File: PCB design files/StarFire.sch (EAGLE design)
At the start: 29 parts, among them U2 ATTINY85-20SU

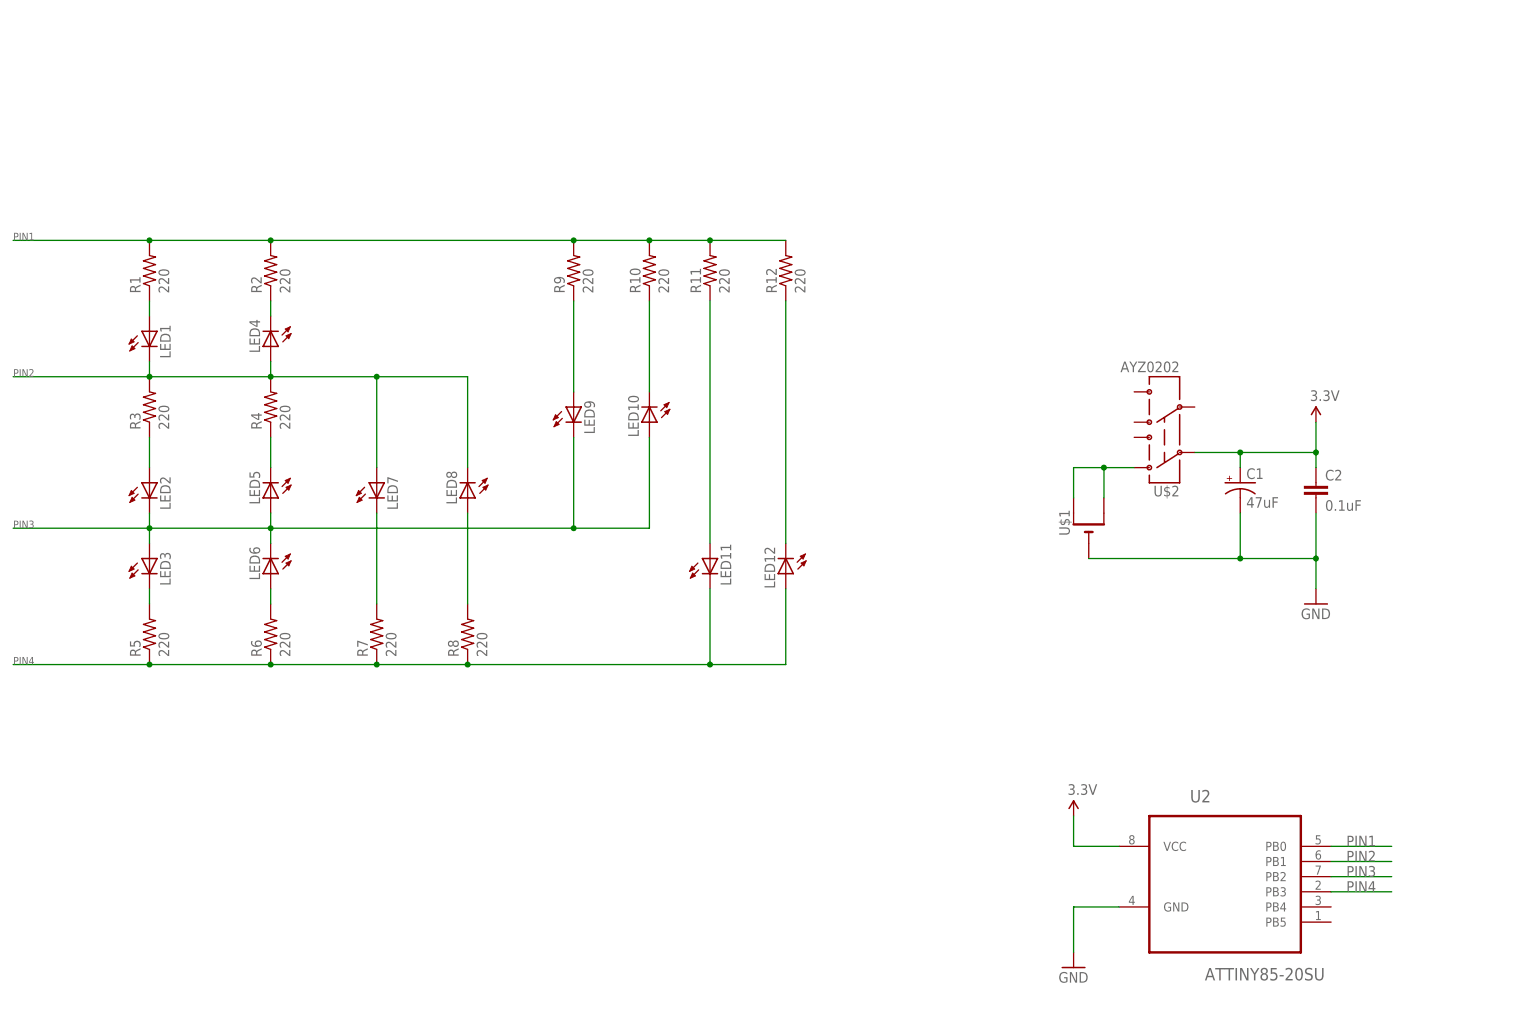
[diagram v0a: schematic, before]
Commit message: cleanup and sort
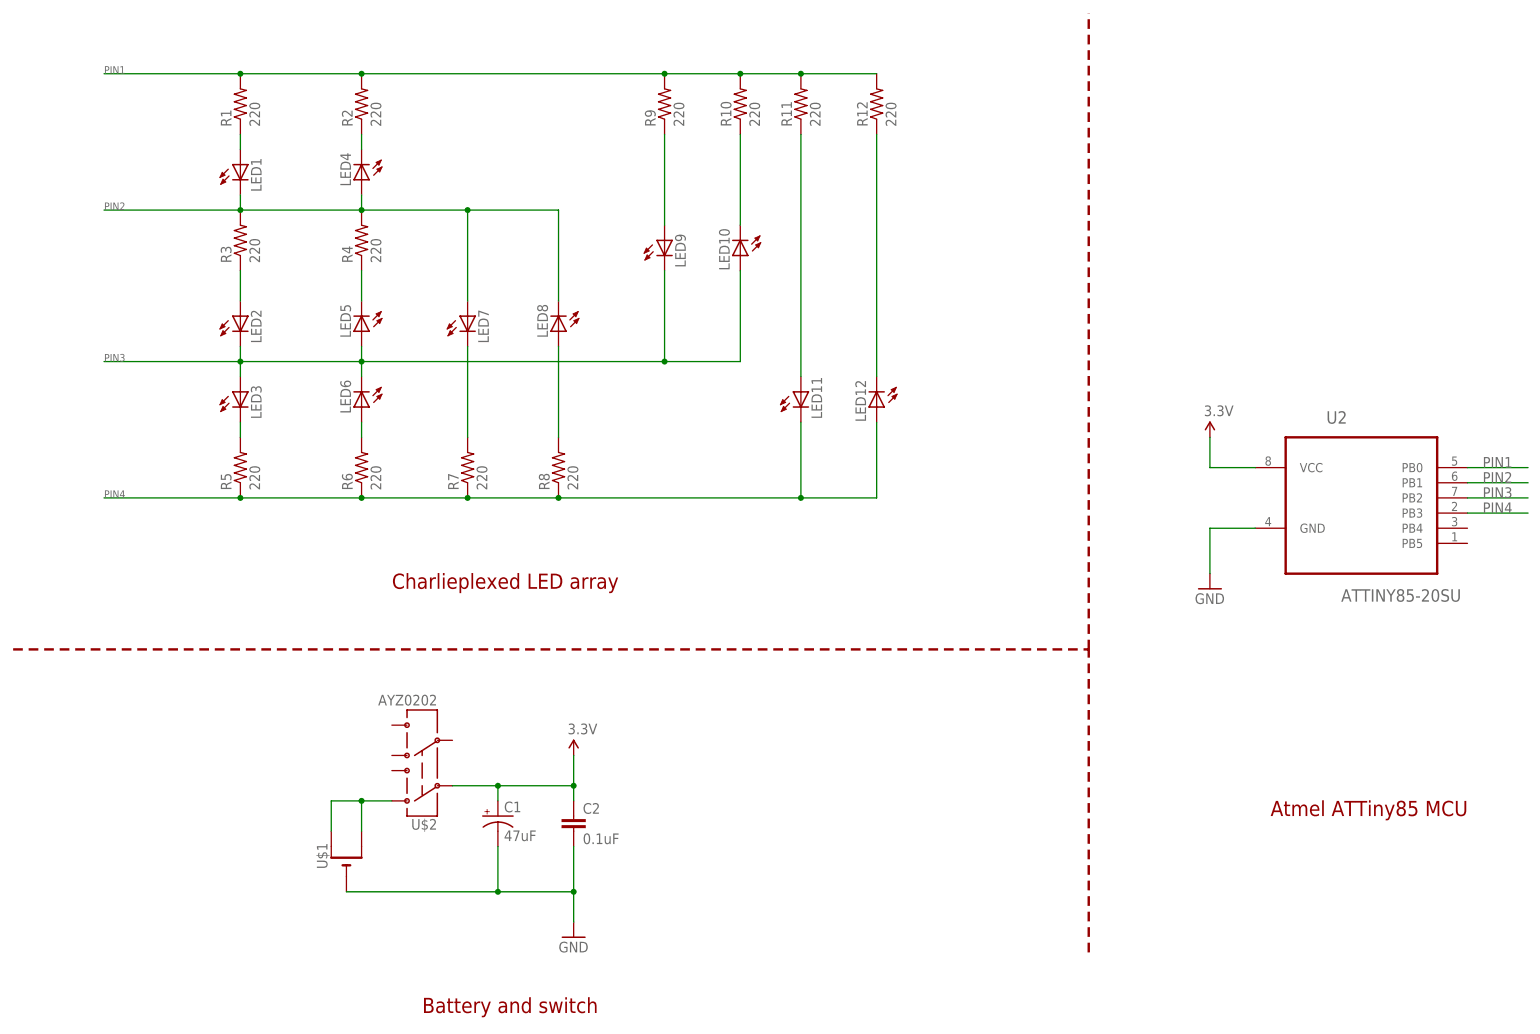
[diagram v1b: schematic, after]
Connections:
- net N$13: now also U$1.+1
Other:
- note added: "Atmel ATTiny85 MCU"
- note added: "Battery and switch"
- note added: "Charlieplexed LED array"
- moved on the sheet: C1, C2, LED1, LED10, LED11, LED12, LED2, LED3, LED4, LED5, LED6, LED7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
